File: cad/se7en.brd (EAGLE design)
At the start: 64.1 x 34 mm, 67 parts, among them CN1 MICROSD-EJECT, CN3 DO NOT PLACE, CN4 DO NOT PLACE, CN5 DO NOT PLACE, CN6 DO NOT PLACE, CN7 DO NOT PLACE, Q1 FDC6329S, SW1 SWITCHKMR211, SW2 SWITCHKMR211, U1 ATSAME70, U2 MCP73831/OT, X1 12MHz, X2 32k768

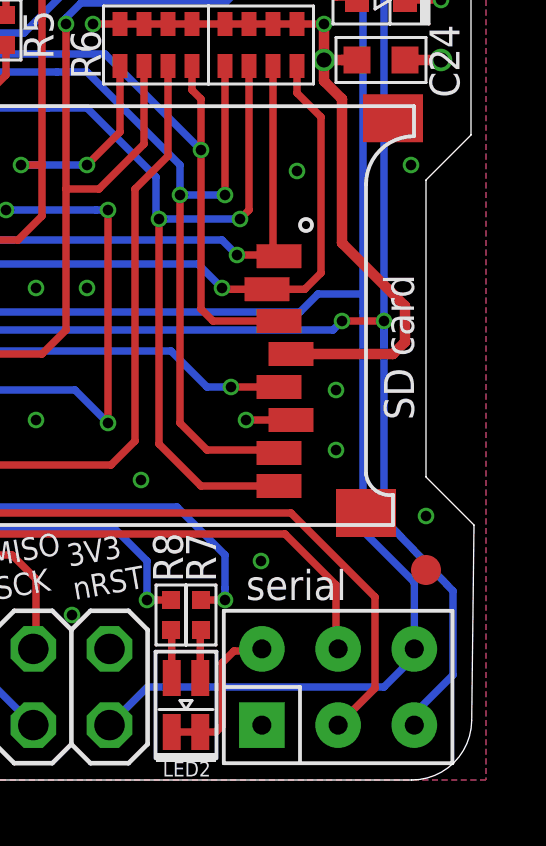
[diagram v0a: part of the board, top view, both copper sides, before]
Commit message: tweak
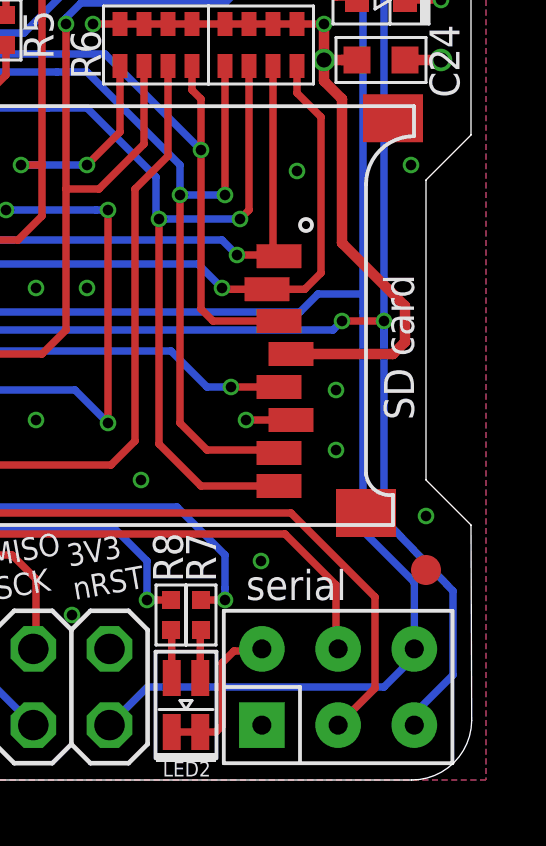
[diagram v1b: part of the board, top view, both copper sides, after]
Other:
- board size 64.1 x 34 mm -> 64 x 34 mm
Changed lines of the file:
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@@
 <grid distance="0.1" unitdist="mm" unit="mm" style="lines" multiple="5" display="yes" altdistance="0.025" altunitdist="inch" altunit="inch"/>
 <layers>
-<layer number="1" name="Top" color="4" fill="1" visible="yes" active="yes"/>
+<layer number="1" name="Top" color="4" fill="1" visible="no" active="yes"/>
 <layer number="2" name="Route2" color="6" fill="1" visible="no" active="yes"/>
 <layer number="3" name="Route3" color="4" fill="3" visible="no" active="no"/>
 <layer number="14" name="Route14" color="1" fill="6" visible="no" active="no"/>
 <layer number="15" name="Route15" color="13" fill="1" visible="no" active="yes"/>
-<layer number="16" name="Bottom" color="1" fill="1" visible="yes" active="yes"/>
+<layer number="16" name="Bottom" color="1" fill="1" visible="no" active="yes"/>
 <layer number="17" name="Pads" color="2" fill="1" visible="yes" active="yes"/>
 <layer number="18" name="Vias" color="2" fill="1" visible="yes" active="yes"/>
@@
 <wire x1="58" y1="35" x2="118.023390625" y2="35" width="0" layer="20"/>
 <wire x1="118.023390625" y1="35" x2="120.023253125" y2="36.976515625" width="0" layer="20" curve="89.327207"/>
-<wire x1="120.023253125" y1="36.976515625" x2="120.1" y2="43.5" width="0" layer="20"/>
-<wire x1="120.1" y1="43.5" x2="118.5" y2="45.1" width="0" layer="20"/>
-<wire x1="118.5" y1="45.1" x2="118.5" y2="55" width="0" layer="20"/>
+<wire x1="120.023253125" y1="36.976515625" x2="120" y2="43.5" width="0" layer="20"/>
+<wire x1="120" y1="43.5" x2="118.5" y2="45" width="0" layer="20"/>
+<wire x1="118.5" y1="45" x2="118.5" y2="55" width="0" layer="20"/>
 <wire x1="118.5" y1="55" x2="120" y2="56.5" width="0" layer="20"/>
 <wire x1="120" y1="56.5" x2="120" y2="67" width="0" layer="20"/>
@@
 <wire x1="67.2" y1="57.2" x2="67.2" y2="56.5" width="0.5" layer="1"/>
 <via x="67.5" y="59" extent="1-16" drill="0.5"/>
-<wire x1="81" y1="56.5" x2="81" y2="56" width="0" layer="19" extent="1-1"/>
 <via x="71.2" y="60" extent="1-16" drill="0.35"/>
 <via x="69.5" y="60.9" extent="1-16" drill="0.35"/>
 <via x="71" y="53.5" extent="1-16" drill="0.35"/>
+<wire x1="81" y1="56.5" x2="81" y2="56" width="0" layer="19" extent="1-1"/>
 </signal>
 <signal name="VCC">

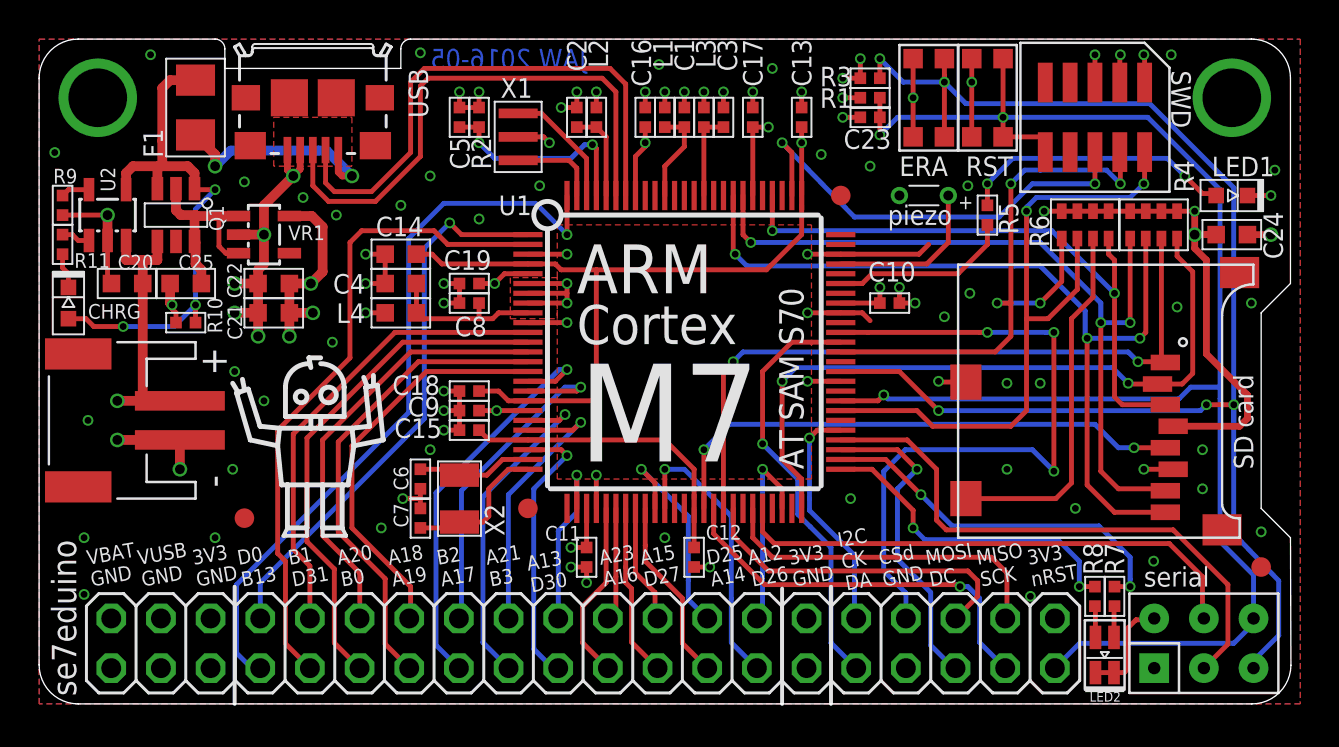
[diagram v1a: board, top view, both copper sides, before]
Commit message: tweak
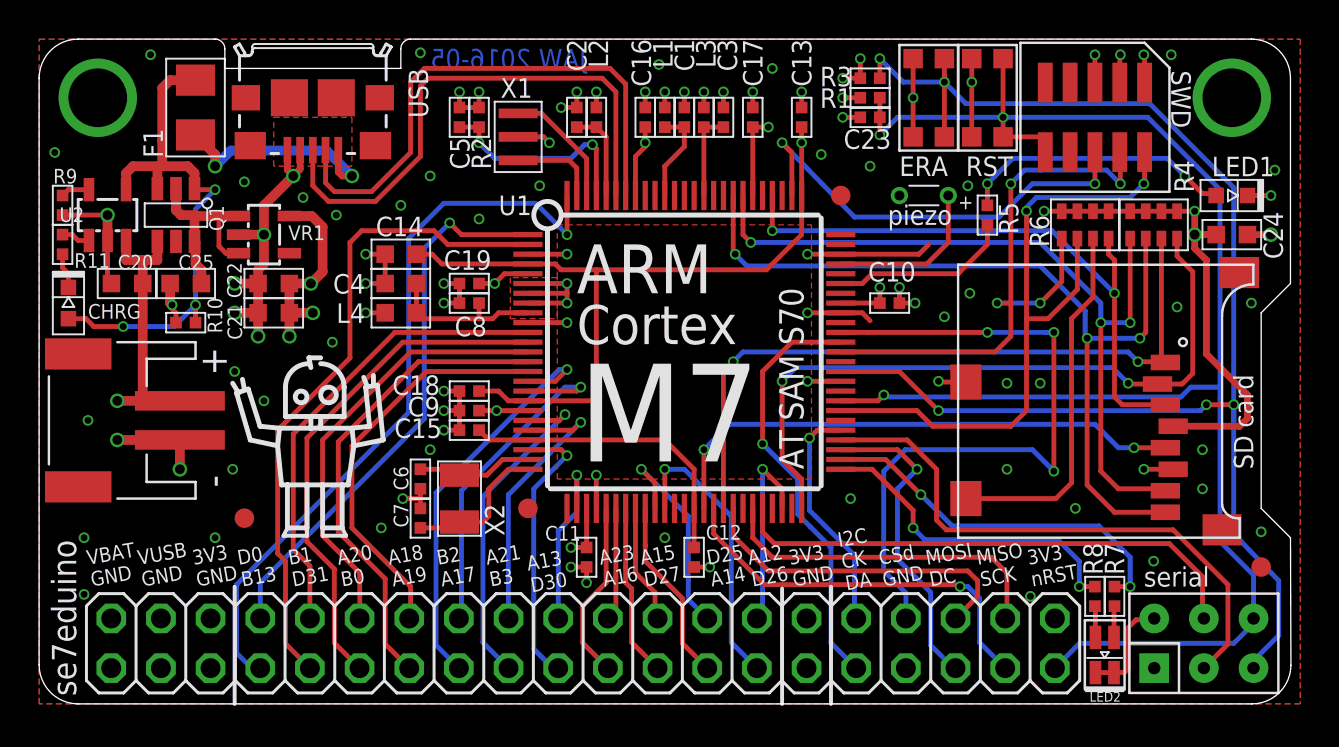
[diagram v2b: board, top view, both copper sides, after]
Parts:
- U2: value MCP73831/OT -> MCP73831; device adafruit:SOT23-5L -> jaw:SOT-23-5
- turned U2 to 90 degrees
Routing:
- net V1V2: track 70.7 -> 71.7 mm
- net IOLED2: track 16.1 -> 16.8 mm
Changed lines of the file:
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@@
 <grid distance="0.1" unitdist="mm" unit="mm" style="lines" multiple="5" display="yes" altdistance="0.025" altunitdist="inch" altunit="inch"/>
 <layers>
-<layer number="1" name="Top" color="4" fill="1" visible="no" active="yes"/>
+<layer number="1" name="Top" color="4" fill="1" visible="yes" active="yes"/>
 <layer number="2" name="Route2" color="6" fill="1" visible="no" active="yes"/>
 <layer number="3" name="Route3" color="4" fill="3" visible="no" active="no"/>
 <layer number="14" name="Route14" color="1" fill="6" visible="no" active="no"/>
 <layer number="15" name="Route15" color="13" fill="1" visible="no" active="yes"/>
-<layer number="16" name="Bottom" color="1" fill="1" visible="no" active="yes"/>
+<layer number="16" name="Bottom" color="1" fill="1" visible="yes" active="yes"/>
 <layer number="17" name="Pads" color="2" fill="1" visible="yes" active="yes"/>
 <layer number="18" name="Vias" color="2" fill="1" visible="yes" active="yes"/>
@@
 <element name="U$3" library="jaw" package="ROBOTMAN-LOGO2" value="ROBOTMAN-LOGO2" x="70.1" y="48"/>
 <element name="LOGO1" library="SparkFun-Aesthetics" package="OSHW-LOGO-M" value="OSHW-LOGOM" x="97.9" y="55.7" rot="MR0"/>
-<element name="U2" library="adafruit" package="SOT23-5L" value="MCP73831/OT" x="59.5" y="60" smashed="yes">
-<attribute name="NAME" x="59.895" y="61.195" size="0.75" layer="25" ratio="10" rot="R90"/>
-<attribute name="VALUE" x="57.595" y="56.571" size="1.27" layer="27"/>
+<element name="U2" library="jaw" package="SOT-23-5" value="MCP73831" x="59.5" y="60" smashed="yes" rot="R90">
+<attribute name="NAME" x="58.305" y="60.395" size="0.75" layer="25" ratio="10" rot="R180"/>
+<attribute name="VALUE" x="62.929" y="58.095" size="1.27" layer="27" rot="R90"/>
 </element>
 <element name="VR1" library="jaw" package="SOT-23-5" value="3v3, 500mA" x="67.5" y="59" smashed="yes">
@@
 <wire x1="81" y1="55.5" x2="83" y2="55.5" width="0.25" layer="1"/>
 <wire x1="81" y1="56" x2="83" y2="56" width="0.25" layer="1"/>
-<wire x1="83" y1="56.5" x2="83" y2="55.5" width="0.25" layer="1"/>
+<wire x1="83" y1="56.5" x2="83" y2="56" width="0.25" layer="1"/>
 <via x="76.7" y="51" extent="1-16" drill="0.35"/>
 <via x="76.7" y="50" extent="1-16" drill="0.35"/>
 <via x="76.7" y="49" extent="1-16" drill="0.35"/>
+<wire x1="83" y1="56" x2="83" y2="55.5" width="0.25" layer="1"/>
 <wire x1="77.5" y1="51" x2="76.7" y2="51" width="0.25" layer="1"/>
 <wire x1="77.5" y1="50" x2="76.7" y2="50" width="0.25" layer="1"/>
@@
 <via x="69.5" y="60.9" extent="1-16" drill="0.35"/>
 <via x="71" y="53.5" extent="1-16" drill="0.35"/>
-<wire x1="81" y1="56.5" x2="81" y2="56" width="0" layer="19" extent="1-1"/>
 </signal>
 <signal name="VCC">
@@
 <wire x1="81" y1="48.5" x2="84.5" y2="48.5" width="0.25" layer="1"/>
 <wire x1="81" y1="50.5" x2="84.5" y2="50.5" width="0.25" layer="1"/>
-<wire x1="89.5" y1="45.5" x2="89.5" y2="47" width="0.25" layer="1"/>
-<wire x1="95" y1="60.5" x2="95" y2="59" width="0.25" layer="1"/>
+<wire x1="89.5" y1="45" x2="89.5" y2="47" width="0.25" layer="1"/>
+<wire x1="95" y1="61" x2="95" y2="59" width="0.25" layer="1"/>
 <via x="84.5" y="66.3" extent="1-16" drill="0.35"/>
 <via x="90" y="66.3" extent="1-16" drill="0.35"/>
@@
 <vertex x="82.5" y="46.5"/>
 </polygon>
-<wire x1="95" y1="60.5" x2="95" y2="61" width="0" layer="19" extent="1-1"/>
-<wire x1="89.5" y1="45" x2="89.5" y2="45.5" width="0" layer="19" extent="1-1"/>
 </signal>
 <signal name="N$2">
@@
 <wire x1="98.9" y1="50.5" x2="99.2" y2="50.8" width="0.25" layer="1"/>
 <via x="99.2" y="50.8" extent="1-16" drill="0.35"/>
-<wire x1="99.2" y1="50.8" x2="99.4" y2="50.6" width="0.25" layer="16"/>
+<wire x1="99.2" y1="50.8" x2="99.5" y2="50.7" width="0.25" layer="16"/>
 <wire x1="99.9" y1="65" x2="99" y2="64.1" width="0.25" layer="16"/>
 <wire x1="99" y1="66" x2="99" y2="65" width="0.25" layer="1"/>
 <wire x1="99" y1="65" x2="99" y2="64.1" width="0.25" layer="1"/>
-<wire x1="99.4" y1="50.6" x2="114.3" y2="50.6" width="0.25" layer="16"/>
-<wire x1="114.3" y1="50.6" x2="114.9" y2="51.2" width="0.25" layer="16"/>
+<wire x1="99.5" y1="50.7" x2="114.4" y2="50.7" width="0.25" layer="16"/>
+<wire x1="114.4" y1="50.7" x2="114.9" y2="51.2" width="0.25" layer="16"/>
 <wire x1="114.9" y1="51.2" x2="116.4" y2="51.2" width="0.25" layer="16"/>
 </signal>
@@
 <wire x1="109.2" y1="41" x2="109.9" y2="41" width="0.25" layer="1"/>
 <wire x1="109.9" y1="41" x2="110" y2="41" width="0.25" layer="1"/>
-<wire x1="97.7" y1="47" x2="98.6" y2="47" width="0.25" layer="1"/>
+<wire x1="97" y1="47" x2="98.6" y2="47" width="0.25" layer="1"/>
 <wire x1="98.6" y1="47" x2="100.7" y2="44.9" width="0.25" layer="1"/>
 <wire x1="100.7" y1="44.9" x2="100.7" y2="44" width="0.25" layer="1"/>
-<wire x1="97.7" y1="47" x2="97" y2="47" width="0" layer="19" extent="1-1"/>
 </signal>
 <signal name="IOLED3">
